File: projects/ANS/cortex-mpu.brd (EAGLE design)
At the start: 34.3 x 40 mm, 66 parts, among them IC1 LM1117MPX-3.3, U1 AT32UC3B164-AUT, Y1 7A-16

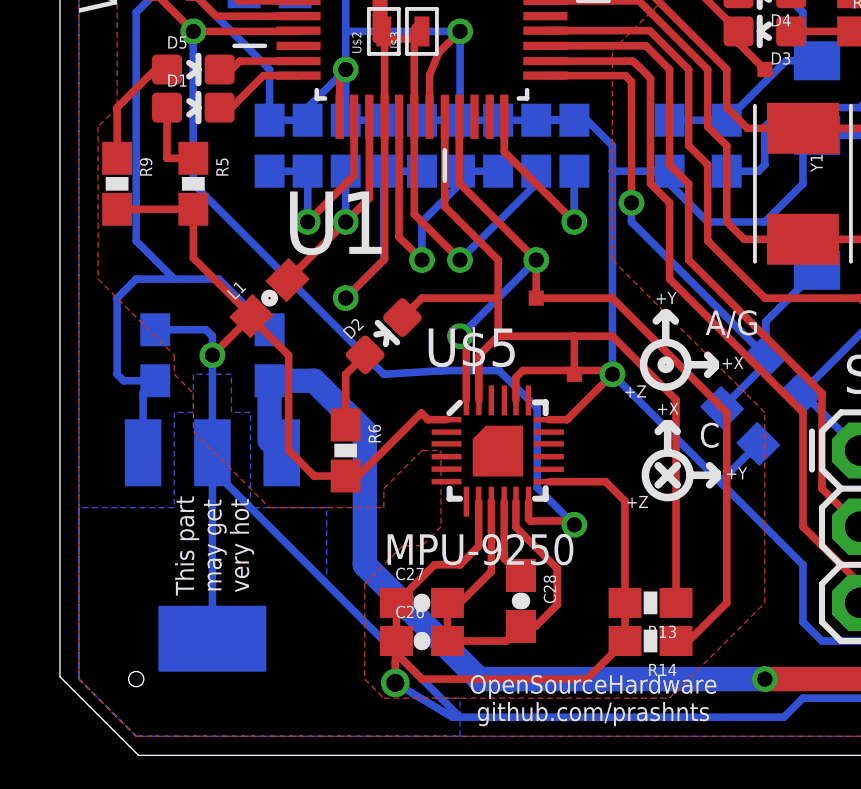
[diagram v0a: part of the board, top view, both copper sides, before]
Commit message: Board Fixes
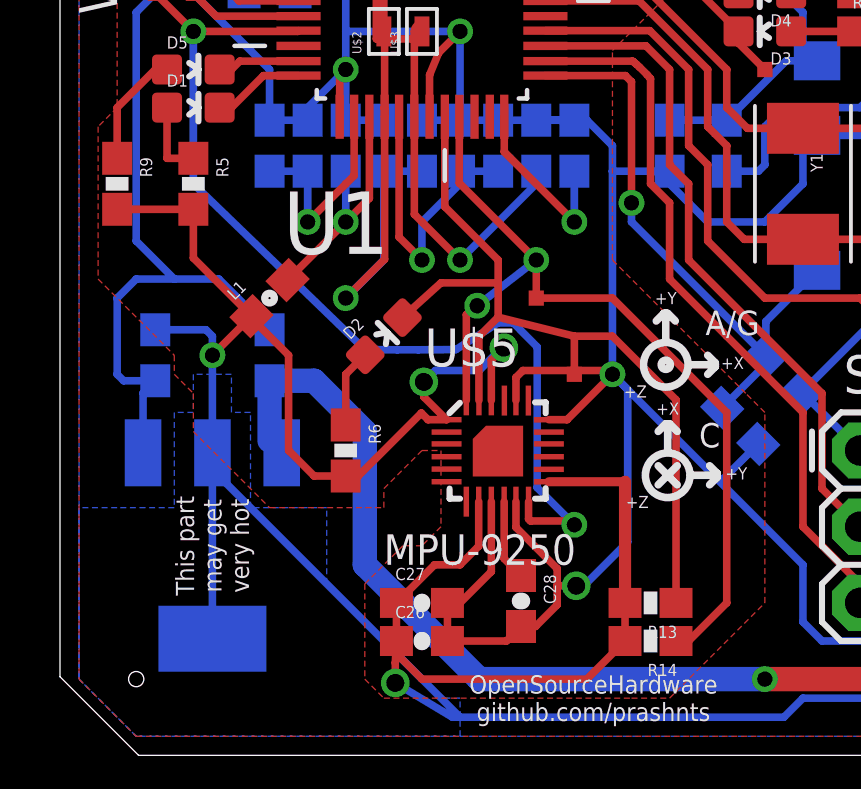
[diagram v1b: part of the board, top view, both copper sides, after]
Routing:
- net GND: track 208.2 -> 216.9 mm, vias 5 -> 6
- net VCC: track 156.9 -> 164.0 mm, vias 4 -> 6
- net PA5: track 31.6 -> 33.3 mm
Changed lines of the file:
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@@
 <contactref element="TP7" pad="P$1"/>
 <via x="24.13" y="5.1435" extent="1-16" drill="0.508"/>
-<wire x1="22.890084375" y1="9.0403625" x2="21.614246875" y2="10.285753125" width="0.254" layer="16"/>
-<wire x1="21.614246875" y1="10.285753125" x2="19.92674375" y2="10.285753125" width="0.254" layer="16"/>
-<wire x1="19.92674375" y1="10.285753125" x2="19.696825" y2="10.278640625" width="0.254" layer="16"/>
-<wire x1="19.696825" y1="10.278640625" x2="19.693146875" y2="10.278471875" width="0.254" layer="16"/>
-<wire x1="19.693146875" y1="10.278471875" x2="17.78" y2="10.16" width="0.254" layer="16"/>
-<wire x1="17.78" y1="10.16" x2="11.43" y2="16.51" width="0.254" layer="16"/>
+<wire x1="22.890084375" y1="11.0723625" x2="22.098" y2="11.8745" width="0.254" layer="16"/>
+<wire x1="22.098" y1="11.8745" x2="21.59" y2="11.8745" width="0.254" layer="16"/>
+<wire x1="21.59" y1="11.8745" x2="20.18074375" y2="10.984253125" width="0.254" layer="16"/>
+<wire x1="20.18074375" y1="10.984253125" x2="18.934825" y2="10.977140625" width="0.254" layer="16"/>
+<wire x1="18.934825" y1="10.977140625" x2="18.232646875" y2="10.976971875" width="0.254" layer="16"/>
+<wire x1="18.232646875" y1="10.976971875" x2="17.145" y2="10.9855" width="0.254" layer="16"/>
+<wire x1="17.145" y1="10.9855" x2="11.43" y2="16.51" width="0.254" layer="16"/>
 <wire x1="11.43" y1="16.51" x2="11.43" y2="21.59" width="0.254" layer="16"/>
 <via x="11.43" y="21.59" extent="1-16" drill="0.508"/>
@@
 <wire x1="22.6695" y1="5.2705" x2="24.003" y2="5.2705" width="0.254" layer="1"/>
 <wire x1="24.003" y1="5.2705" x2="24.13" y2="5.1435" width="0.254" layer="1"/>
-<wire x1="22.890084375" y1="9.0403625" x2="22.890084375" y2="6.383415625" width="0.254" layer="16"/>
+<wire x1="22.890084375" y1="11.0723625" x2="22.890084375" y2="6.383415625" width="0.254" layer="16"/>
 <wire x1="22.890084375" y1="6.383415625" x2="24.13" y2="5.1435" width="0.254" layer="16"/>
 </signal>
@@
 <wire x1="19.812" y1="18.7452" x2="19.812" y2="15.748" width="0.254" layer="1"/>
 <wire x1="19.812" y1="15.748" x2="21.59" y2="13.97" width="0.254" layer="1"/>
-<wire x1="21.59" y1="11.43" x2="24.13" y2="11.43" width="0.254" layer="1"/>
+<wire x1="21.59" y1="12.065" x2="24.13" y2="11.43" width="0.254" layer="1"/>
 <wire x1="24.13" y1="11.43" x2="25.4" y2="11.43" width="0.254" layer="1"/>
 <wire x1="27.52" y1="2.54" x2="27.52" y2="9.31" width="0.254" layer="1"/>
 <wire x1="27.52" y1="9.31" x2="25.4" y2="11.43" width="0.254" layer="1"/>
 <wire x1="24.13" y1="10.16" x2="24.13" y2="11.43" width="0.254" layer="1"/>
-<wire x1="21.59" y1="13.97" x2="21.59" y2="12.7" width="0.254" layer="1"/>
-<wire x1="21.59" y1="12.7" x2="21.59" y2="11.43" width="0.254" layer="1"/>
-<wire x1="18.40013125" y1="12.05013125" x2="19.05" y2="12.7" width="0.254" layer="1"/>
-<wire x1="19.05" y1="12.7" x2="21.59" y2="12.7" width="0.254" layer="1"/>
-<wire x1="20.94936875" y1="9.29133125" x2="20.94936875" y2="10.78936875" width="0.254" layer="1"/>
-<wire x1="20.94936875" y1="10.78936875" x2="21.59" y2="11.43" width="0.254" layer="1"/>
+<wire x1="21.59" y1="13.97" x2="21.59" y2="13.208" width="0.254" layer="1"/>
+<wire x1="21.59" y1="13.208" x2="21.59" y2="12.065" width="0.254" layer="1"/>
+<wire x1="18.40013125" y1="12.05013125" x2="19.685" y2="13.208" width="0.254" layer="1"/>
+<wire x1="19.685" y1="13.208" x2="21.59" y2="13.208" width="0.254" layer="1"/>
+<wire x1="20.94936875" y1="9.29133125" x2="20.94936875" y2="11.42436875" width="0.254" layer="1"/>
+<wire x1="20.94936875" y1="11.42436875" x2="21.59" y2="12.065" width="0.254" layer="1"/>
 </signal>
 <signal name="PA10">
@@
 <wire x1="20.2946" y1="18.7452" x2="20.2946" y2="16.5354" width="0.254" layer="1"/>
 <wire x1="20.2946" y1="16.5354" x2="22.86" y2="13.97" width="0.254" layer="1"/>
-<wire x1="20.34" y1="11.41" x2="20.32" y2="11.43" width="0.254" layer="1"/>
-<via x="20.32" y="11.43" extent="1-16" drill="0.508"/>
+<via x="20.8915" y="12.446" extent="1-16" drill="0.508"/>
 <via x="22.86" y="13.97" extent="1-16" drill="0.508"/>
-<wire x1="22.86" y1="13.97" x2="20.32" y2="11.43" width="0.254" layer="16"/>
+<wire x1="22.86" y1="13.97" x2="20.8915" y2="12.446" width="0.254" layer="16"/>
 <wire x1="22.86" y1="12.7" x2="22.86" y2="13.97" width="0.254" layer="1"/>
 <wire x1="22.86" y1="12.7" x2="25.4" y2="12.7" width="0.254" layer="1"/>
@@
 <wire x1="27.94" y1="1.27" x2="29.21" y2="2.54" width="0.254" layer="1"/>
 <wire x1="29.21" y1="2.54" x2="29.21" y2="8.89" width="0.254" layer="1"/>
-<wire x1="20.529053125" y1="9.29133125" x2="20.529053125" y2="11.220946875" width="0.254" layer="1"/>
-<wire x1="20.529053125" y1="11.220946875" x2="20.32" y2="11.43" width="0.254" layer="1"/>
+<wire x1="20.529053125" y1="9.29133125" x2="20.529053125" y2="12.147053125" width="0.254" layer="1"/>
+<wire x1="20.529053125" y1="12.147053125" x2="20.8915" y2="12.446" width="0.254" layer="1"/>
 </signal>
 <signal name="PA11">
@@
 <vertex x="7.62" y="0"/>
 </polygon>
-<polygon width="0.254" layer="1" spacing="0.3048" isolate="0.4064" orphans="yes" rank="3">
+<polygon width="0.254" layer="1" spacing="0.3048" isolate="0.4064" rank="3">
 <vertex x="9.525" y="34.29"/>
 <vertex x="7.62" y="32.385"/>
@@
 <wire x1="22.4155" y1="10.287" x2="25.273" y2="10.287" width="0.254" layer="1"/>
 <wire x1="25.273" y1="10.287" x2="25.4" y2="10.16" width="0.254" layer="1"/>
-<wire x1="22.183228125" y1="5.914809375" x2="22.183228125" y2="5.058271875" width="0.254" layer="1"/>
-<wire x1="22.183228125" y1="5.058271875" x2="23.5585" y2="3.683" width="0.254" layer="1"/>
-<wire x1="23.5585" y1="3.683" x2="23.5585" y2="2.4765" width="0.254" layer="1"/>
+<wire x1="23.5585" y1="3.1115" x2="23.5585" y2="2.4765" width="0.254" layer="1"/>
 <wire x1="19.9" y1="1.27" x2="21.8685" y2="1.27" width="0.254" layer="1"/>
 <wire x1="21.8685" y1="1.27" x2="22.352" y2="1.7535" width="0.254" layer="1"/>
@@
 <wire x1="22.8355" y1="1.7535" x2="22.352" y2="1.7535" width="0.254" layer="1"/>
 <wire x1="20.32" y1="2.54" x2="19.9" y2="2.54" width="0.254" layer="1"/>
-<wire x1="23.28165" y1="8.6470875" x2="22.183228125" y2="5.914809375" width="0" layer="19" extent="1-1"/>
-<wire x1="36.41" y1="17.78" x2="35.27" y2="18.125" width="0" layer="19" extent="1-16"/>
+<wire x1="22.183228125" y1="5.914809375" x2="22.183228125" y2="5.058271875" width="0.254" layer="1"/>
+<wire x1="22.183228125" y1="5.058271875" x2="23.5585" y2="3.683" width="0.254" layer="1"/>
+<wire x1="23.5585" y1="3.683" x2="23.5585" y2="3.1115" width="0.254" layer="1"/>
+<wire x1="23.5585" y1="3.1115" x2="24.1935" y2="3.1115" width="0.254" layer="1"/>
+<via x="24.1935" y="3.1115" extent="1-16" drill="0.6"/>
+<wire x1="24.1935" y1="3.1115" x2="24.4475" y2="3.1115" width="0.254" layer="16"/>
+<wire x1="24.4475" y1="3.1115" x2="25.908" y2="4.572" width="0.254" layer="16"/>
+<wire x1="25.908" y1="4.572" x2="25.908" y2="9.652" width="0.254" layer="16"/>
+<wire x1="25.908" y1="9.652" x2="25.4" y2="10.16" width="0.254" layer="16"/>
+<wire x1="35.27" y1="18.125" x2="36.41" y2="17.78" width="0" layer="19" extent="1-16"/>
 </signal>
 <signal name="VBUS">
@@
 <wire x1="19.05" y1="0" x2="17.78" y2="1.27" width="0.254" layer="1"/>
 <wire x1="17.78" y1="1.27" x2="18.2" y2="1.27" width="0.254" layer="1"/>
-<wire x1="25.82" y1="5.93" x2="25.17063125" y2="6.57936875" width="0.254" layer="1"/>
-<wire x1="25.82" y1="5.93" x2="25.82" y2="2.54" width="0.254" layer="1"/>
 <wire x1="25.82" y1="2.54" x2="25.82" y2="1.27" width="0.254" layer="1"/>
 <wire x1="19.05" y1="0" x2="24.55" y2="0" width="0.254" layer="1"/>
@@
 </polygon>
 <wire x1="20.94259375" y1="5.914809375" x2="20.94259375" y2="4.43259375" width="0.254" layer="1"/>
-<wire x1="23.281646875" y1="6.57936875" x2="25.17063125" y2="6.57936875" width="0.254" layer="1"/>
 <wire x1="19.871265625" y1="8.6470875" x2="19.2529125" y2="8.6470875" width="0.254" layer="1"/>
 <wire x1="19.2529125" y1="8.6470875" x2="19.03" y2="8.87" width="0.254" layer="1"/>
@@
 <wire x1="18.161" y1="-0.127" x2="18.161" y2="0.547" width="0.254" layer="1"/>
 <wire x1="18.161" y1="0.547" x2="18.2" y2="1.27" width="0.254" layer="1"/>
-<wire x1="19.871265625" y1="8.6470875" x2="21.3629125" y2="9.29133125" width="0" layer="19" extent="1-1"/>
+<wire x1="23.281646875" y1="6.57936875" x2="25.82" y2="6.57936875" width="0.3048" layer="1"/>
+<wire x1="25.82" y1="6.57936875" x2="25.82" y2="2.54" width="0.4064" layer="1"/>
+<wire x1="21.3629125" y1="9.29133125" x2="21.3629125" y2="10.6314125" width="0.254" layer="1"/>
+<wire x1="21.3629125" y1="10.6314125" x2="21.7805" y2="11.049" width="0.254" layer="1"/>
+<via x="21.7805" y="11.049" extent="1-16" drill="0.6"/>
+<wire x1="21.7805" y1="11.049" x2="21.717" y2="11.049" width="0.254" layer="16"/>
+<wire x1="21.717" y1="11.049" x2="20.955" y2="10.287" width="0.254" layer="16"/>
+<wire x1="20.955" y1="10.287" x2="19.4945" y2="10.287" width="0.254" layer="16"/>
+<wire x1="19.4945" y1="10.287" x2="19.1135" y2="9.906" width="0.254" layer="16"/>
+<via x="19.1135" y="9.906" extent="1-16" drill="0.6"/>
+<wire x1="19.1135" y1="9.906" x2="19.1135" y2="9.404853125" width="0.254" layer="1"/>
+<wire x1="19.1135" y1="9.404853125" x2="19.871265625" y2="8.6470875" width="0.254" layer="1"/>
 </signal>
 <signal name="N$5">
